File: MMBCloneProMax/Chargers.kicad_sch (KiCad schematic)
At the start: 8 parts, among them J6 Current Sense, J7 Bat1, U2 LTC4054ES5-4.2

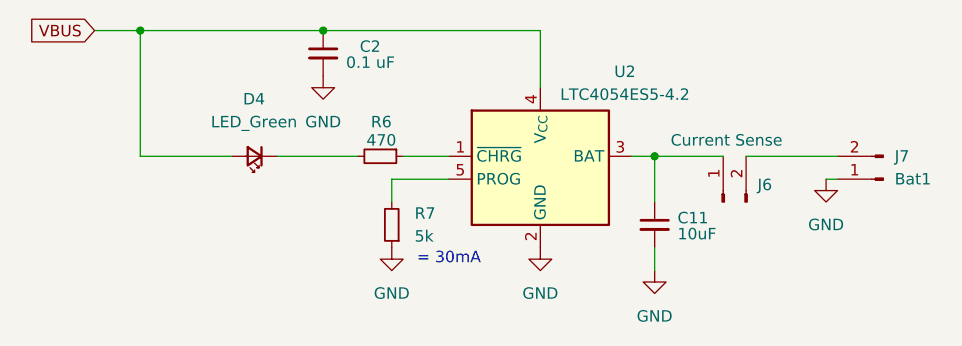
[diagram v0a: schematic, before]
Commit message: drc done
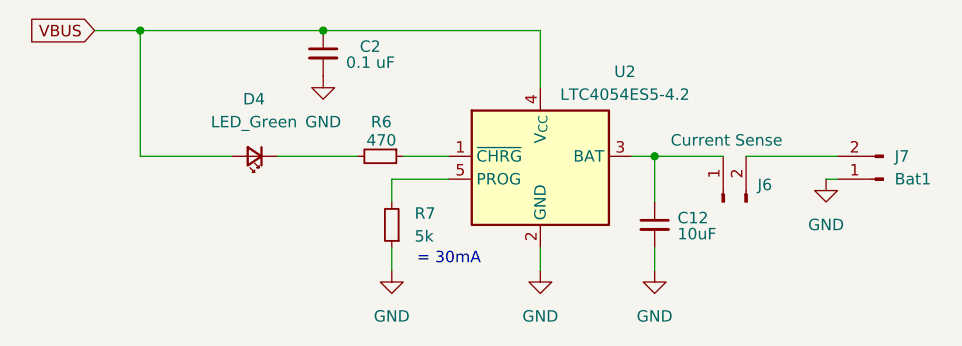
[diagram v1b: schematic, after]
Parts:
- renumbered C11 to C12
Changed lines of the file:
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@@
+	(wire
+		(pts
+			(xy 137.16 81.28) (xy 137.16 78.74)
+		)
+		(stroke
+			(width 0)
+			(type default)
+		)
+	)
 	(wire
 		(pts
@@
 		(pts
 			(xy 143.51 71.12) (xy 137.16 71.12)
+		)
+		(stroke
+			(width 0)
+			(type default)
+		)
+	)
+	(wire
+		(pts
+			(xy 153.67 81.28) (xy 153.67 78.74)
 		)
 		(stroke
@@
 		(on_board yes)
 		(dnp no)
-		(property "Reference" "C11"
+		(property "Reference" "C12"
 			(at 168.91 75.438 0)
 			(effects
@@
 	(symbol
 		(lib_id "power:GND")
-		(at 153.67 78.74 0)
+		(at 153.67 81.28 0)
 		(unit 1)
 		(exclude_from_sim no)
@@
 		(fields_autoplaced yes)
 		(property "Reference" "#PWR012"
-			(at 153.67 85.09 0)
+			(at 153.67 87.63 0)
 			(effects
 				(font
@@
 		)
 		(property "Value" "GND"
-			(at 153.67 83.82 0)
+			(at 153.67 86.36 0)
 			(effects
 				(font
@@
 		)
 		(property "Footprint" ""
-			(at 153.67 78.74 0)
+			(at 153.67 81.28 0)
 			(effects
 				(font
@@
 		)
 		(property "Datasheet" ""
-			(at 153.67 78.74 0)
+			(at 153.67 81.28 0)
 			(effects
 				(font
@@
 		)
 		(property "Description" "Power symbol creates a global label with name \"GND\" , ground"
-			(at 153.67 78.74 0)
+			(at 153.67 81.28 0)
 			(effects
 				(font
@@
 	(symbol
 		(lib_id "power:GND")
-		(at 137.16 78.74 0)
+		(at 137.16 81.28 0)
 		(unit 1)
 		(exclude_from_sim no)
@@
 		(fields_autoplaced yes)
 		(property "Reference" "#PWR011"
-			(at 137.16 85.09 0)
+			(at 137.16 87.63 0)
 			(effects
 				(font
@@
 		)
 		(property "Value" "GND"
-			(at 137.16 83.82 0)
+			(at 137.16 86.36 0)
 			(effects
 				(font
@@
 		)
 		(property "Footprint" ""
-			(at 137.16 78.74 0)
+			(at 137.16 81.28 0)
 			(effects
 				(font
@@
 		)
 		(property "Datasheet" ""
-			(at 137.16 78.74 0)
+			(at 137.16 81.28 0)
 			(effects
 				(font
@@
 		)
 		(property "Description" "Power symbol creates a global label with name \"GND\" , ground"
-			(at 137.16 78.74 0)
+			(at 137.16 81.28 0)
 			(effects
 				(font
@@
 		(dnp no)
 		(fields_autoplaced yes)
-		(property "Reference" "#PWR046"
+		(property "Reference" "#PWR047"
 			(at 166.37 87.63 0)
 			(effects
